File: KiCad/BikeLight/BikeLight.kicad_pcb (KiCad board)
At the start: 2 copper layers, 170.5 x 50 mm, 64 parts, among them J1 Conn-01x02_P2.5mm_S2B-XH-A-BK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, J2 Conn-01x02_P2.5mm_S2B-XH-A-BK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, J3 GT-USB-7051A, J4 Conn-01x02_P2.5mm_S2B-XH-A-BK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, J5 Conn-01x02_P2.5mm_S2B-XH-A-BK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, J6 Conn_01x05, Q1 AO3401A, Q2 AO3400A, Q3 BC847BDW1, SW2 SW_PB_B3F-4055, SW3 K2-1102AQ-H4CW-01, U1 TP4056-42-ESOP8, U2 MPU-6050, U3 MAX17048, U4 MCP1826S-33, U5 RFID-RC522, U6 MT3608, U8 HT-CT62

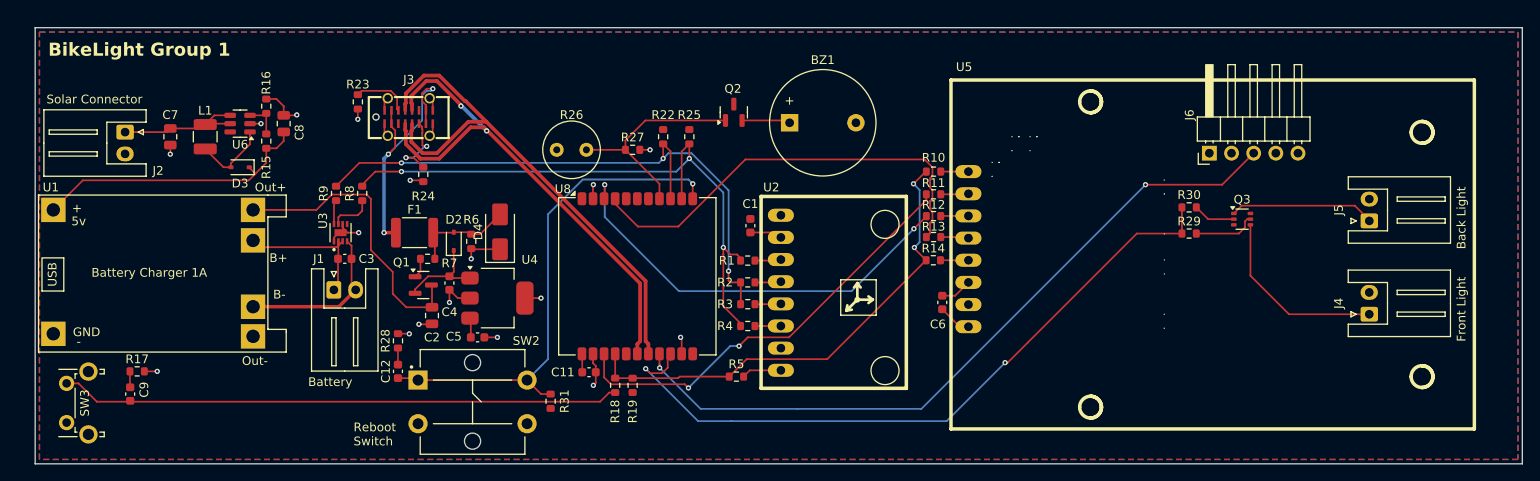
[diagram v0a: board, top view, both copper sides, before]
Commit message: Cleanup and created new fabrication files
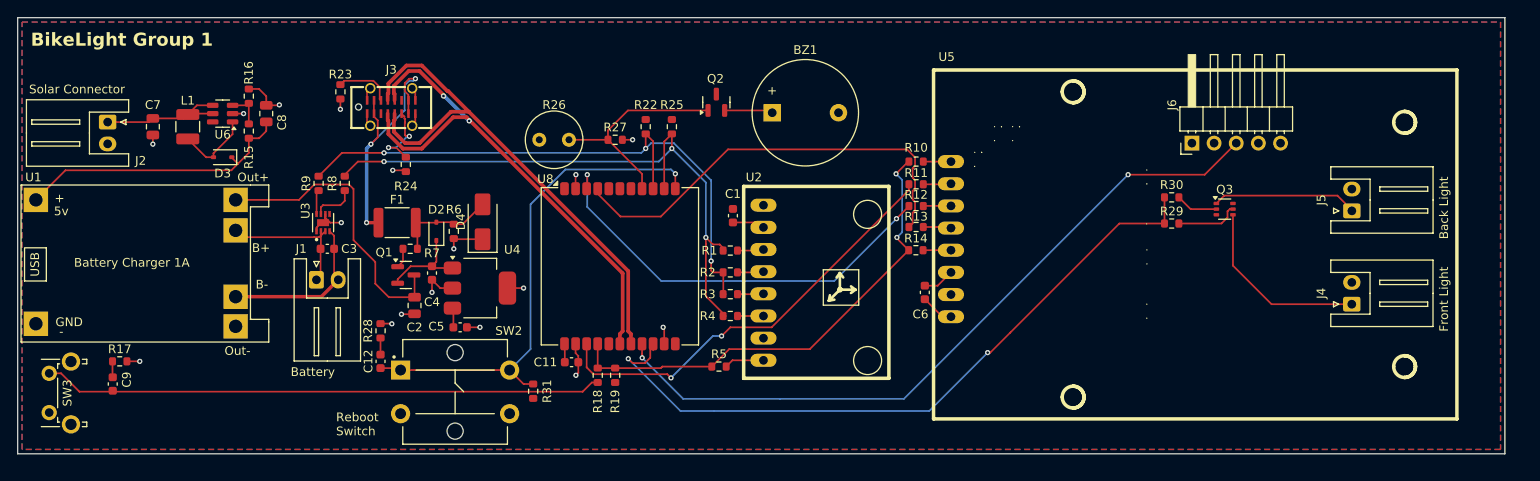
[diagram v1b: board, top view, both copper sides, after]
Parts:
- moved C11 2.31 mm to (83.0, 69.0)
- moved C5 2.31 mm to (70.2, 65.0)
- moved C9 2.31 mm to (30.4, 71.5)
- moved R14 2.31 mm to (122.4, 56.2)
- moved R18 2.31 mm to (86.0, 70.5)
- moved R19 2.31 mm to (88.0, 70.5)
- moved R5 2.31 mm to (99.8, 69.5)
- moved U2 2.31 mm to (103.2, 70.8)
- moved BZ1 2.31 mm to (106.0, 40.4)
- moved C1 2.31 mm to (101.5, 52.2)
- moved C2 2.31 mm to (65.0, 62.5)
- moved C3 2.31 mm to (55.0, 56.0)
- moved C4 2.31 mm to (67.0, 58.8)
- moved C6 2.31 mm to (123.4, 61.0)
- moved C7 2.31 mm to (35.0, 42.0)
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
